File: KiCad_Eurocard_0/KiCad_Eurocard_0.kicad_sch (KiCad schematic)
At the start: 137 parts, among them IC1 ADF4351BCPZ, IC1 ADP3334ARZ, IC2 AD9959BCPZ, IC2 CY7C68013A-56LTX, J1 Conn_Coaxial, J2 Conn_Coaxial, J3 Conn_Coaxial, J4 Conn_Coaxial, J5 Conn_Coaxial, J6 Conn_Coaxial, J7 Conn_Coaxial, J8 Conn_Coaxial, J9 USB_B_Mini, SW1 SW_DIP_x01, SW2 SW_DIP_x01, U1 ADP150ACBZ-2.85R7, U2 ADP150ACBZ-2.85R7, U4 24LC64, Y1 ECS-240-12-20A-TR

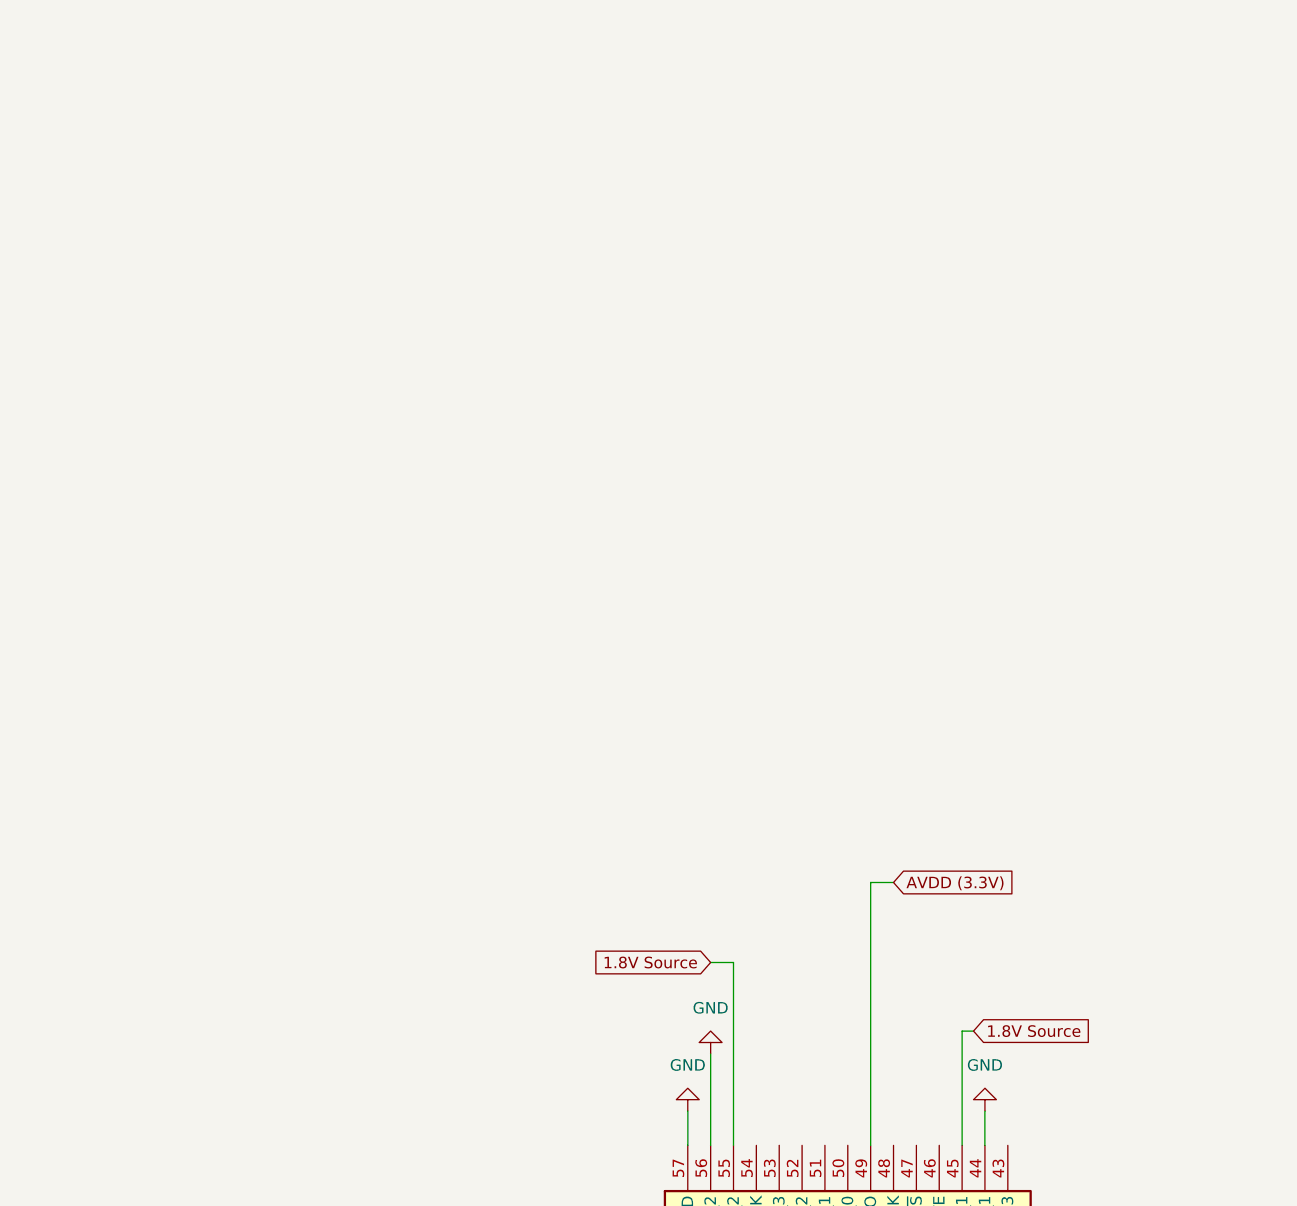
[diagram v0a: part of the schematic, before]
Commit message: Update KiCad_Eurocard_0.kicad_sch
test1000
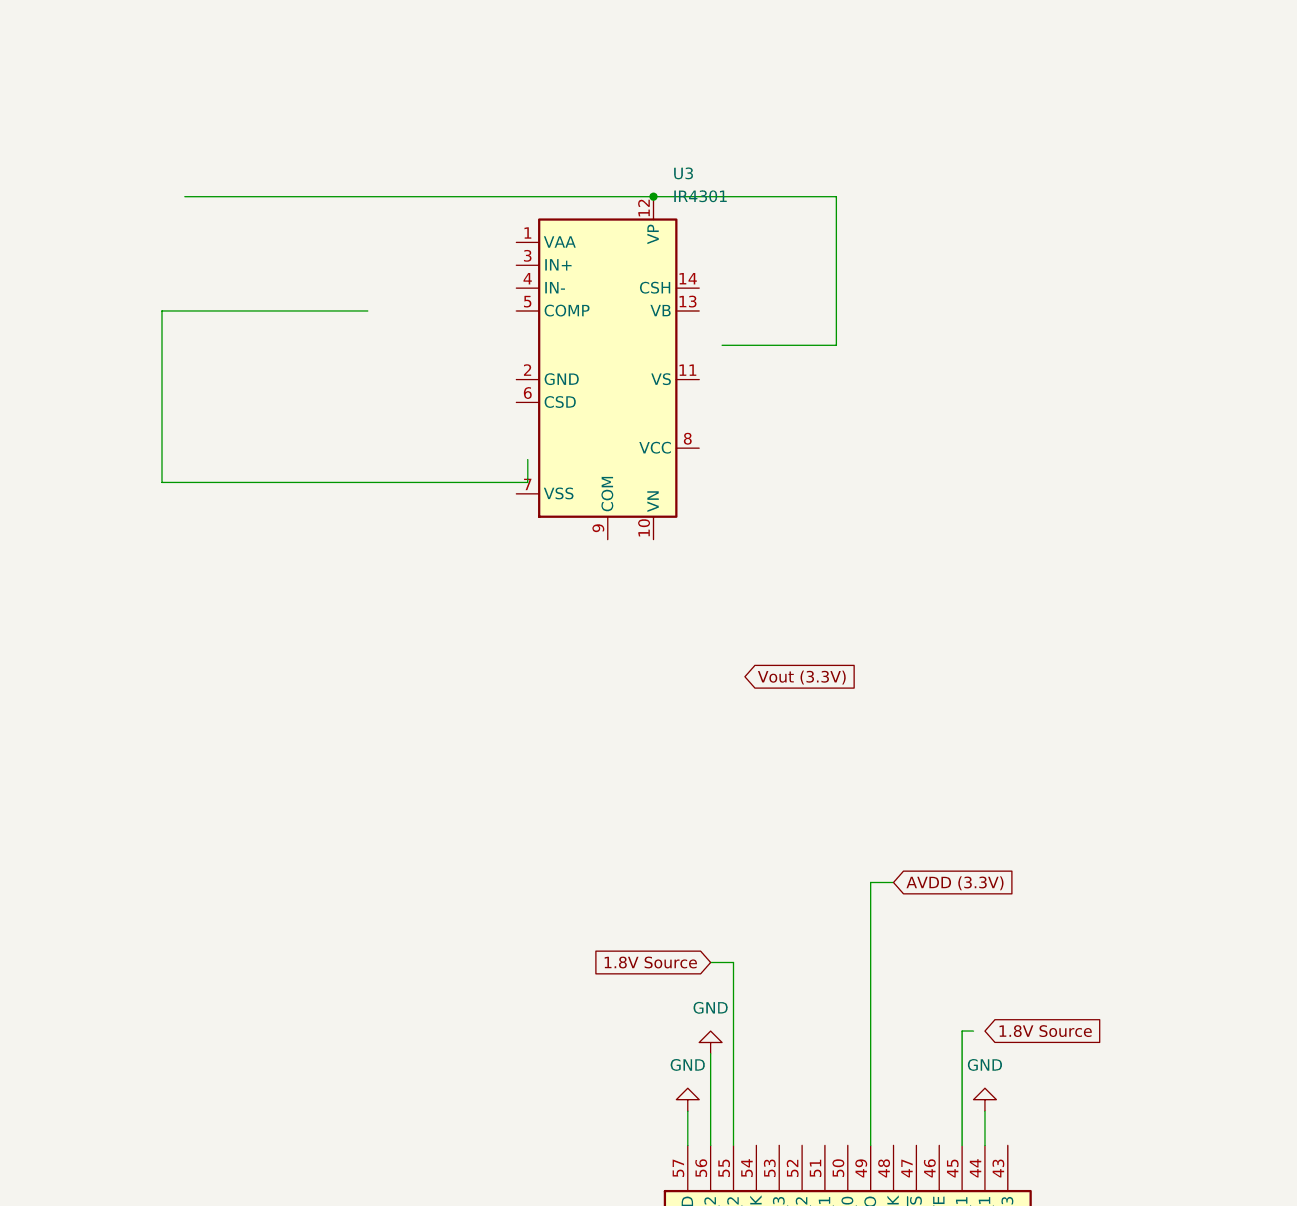
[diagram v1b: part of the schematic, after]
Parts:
- added U3: IR4301, Package_DFN_QFN:Infineon_PQFN-22-15-4EP_6x5mm_P0.65mm, symbol Amplifier_Audio:IR4301
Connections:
- net 1.8V Source: no longer IC2.45 (DVDD_1)
- new net: U3.15 (COM), U3.9 (COM)
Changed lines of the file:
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@@
 	)
 	(junction
+		(at 311.15 163.83)
+		(diameter 0)
+		(color 0 0 0 0)
+	)
+	(junction
 		(at 46.99 227.33)
 		(diameter 0)
@@
 	(wire
 		(pts
+			(xy 297.18 193.04) (xy 297.18 195.58)
+		)
+		(stroke
+			(width 0)
+			(type default)
+		)
+	)
+	(wire
+		(pts
 			(xy 306.07 367.03) (xy 306.07 368.3)
 		)
@@
 	(wire
 		(pts
+			(xy 279.4 176.53) (xy 256.54 176.53)
+		)
+		(stroke
+			(width 0)
+			(type default)
+		)
+	)
+	(wire
+		(pts
 			(xy 459.74 279.4) (xy 459.74 278.13)
 		)
@@
 	(wire
 		(pts
+			(xy 331.47 163.83) (xy 331.47 180.34)
+		)
+		(stroke
+			(width 0)
+			(type default)
+		)
+	)
+	(wire
+		(pts
 			(xy 115.57 107.95) (xy 128.27 107.95)
 		)
@@
 	(wire
 		(pts
+			(xy 256.54 176.53) (xy 256.54 195.58)
+		)
+		(stroke
+			(width 0)
+			(type default)
+		)
+	)
+	(wire
+		(pts
 			(xy 185.42 219.71) (xy 181.61 219.71)
 		)
@@
 	(wire
 		(pts
+			(xy 256.54 195.58) (xy 297.18 195.58)
+		)
+		(stroke
+			(width 0)
+			(type default)
+		)
+	)
+	(wire
+		(pts
 			(xy 85.09 227.33) (xy 85.09 234.95)
 		)
@@
 	(wire
 		(pts
+			(xy 311.15 163.83) (xy 331.47 163.83)
+		)
+		(stroke
+			(width 0)
+			(type default)
+		)
+	)
+	(wire
+		(pts
 			(xy 527.05 182.88) (xy 527.05 187.96)
 		)
@@
 	(wire
 		(pts
+			(xy 259.08 163.83) (xy 311.15 163.83)
+		)
+		(stroke
+			(width 0)
+			(type default)
+		)
+	)
+	(wire
+		(pts
 			(xy 485.14 22.86) (xy 499.11 22.86)
 		)
@@
 	(wire
 		(pts
+			(xy 318.77 180.34) (xy 331.47 180.34)
+		)
+		(stroke
+			(width 0)
+			(type default)
+		)
+	)
+	(wire
+		(pts
 			(xy 378.46 83.82) (xy 378.46 92.71)
 		)
@@
 		)
 	)
+	(global_label "Vout (3.3V)"
+		(shape input)
+		(at 321.31 217.17 0)
+		(fields_autoplaced yes)
+		(effects
+			(font
+				(size 1.27 1.27)
+			)
+			(justify left)
+		)
+		(property "Intersheetrefs" "${INTERSHEET_REFS}"
+			(at 335.1809 217.17 0)
+			(effects
+				(font
+					(size 1.27 1.27)
+				)
+				(justify left)
+				(hide yes)
+			)
+		)
+	)
 	(global_label "A2 OUT"
 		(shape input)
@@
 	(global_label "1.8V Source"
 		(shape input)
-		(at 346.71 256.54 0)
+		(at 347.98 256.54 0)
 		(fields_autoplaced yes)
 		(effects
@@
 		)
 		(property "Intersheetrefs" "${INTERSHEET_REFS}"
-			(at 361.2461 256.54 0)
+			(at 362.5161 256.54 0)
 			(effects
 				(font
@@
 		)
 		(instances
-			(project ""
+			(project "KiCad_Eurocard_0"
 				(path "/9cb3cf89-0e72-4eef-94e8-d924ebdf2eea"
 					(reference "IC1")
@@
 		)
 		(instances
-			(project ""
+			(project "KiCad_Eurocard_0"
 				(path "/9cb3cf89-0e72-4eef-94e8-d924ebdf2eea"
 					(reference "SW1")
@@
 		)
 		(instances
-			(project ""
+			(project "KiCad_Eurocard_0"
 				(path "/9cb3cf89-0e72-4eef-94e8-d924ebdf2eea"
 					(reference "#PWR06")
@@
 		)
 		(instances
-			(project ""
+			(project "KiCad_Eurocard_0"
 				(path "/9cb3cf89-0e72-4eef-94e8-d924ebdf2eea"
 					(reference "R39")
@@
 		)
 		(instances
-			(project ""
+			(project "KiCad_Eurocard_0"
 				(path "/9cb3cf89-0e72-4eef-94e8-d924ebdf2eea"
 					(reference "J9")
@@
 		)
 		(instances
-			(project ""
+			(project "KiCad_Eurocard_0"
 				(path "/9cb3cf89-0e72-4eef-94e8-d924ebdf2eea"
 					(reference "J1")
@@
 		)
 		(instances
-			(project ""
+			(project "KiCad_Eurocard_0"
 				(path "/9cb3cf89-0e72-4eef-94e8-d924ebdf2eea"
 					(reference "IC2")
@@
 		)
 		(instances
-			(project ""
+			(project "KiCad_Eurocard_0"
 				(path "/9cb3cf89-0e72-4eef-94e8-d924ebdf2eea"
 					(reference "#PWR035")
@@
 		)
 		(instances
-			(project ""
+			(project "KiCad_Eurocard_0"
 				(path "/9cb3cf89-0e72-4eef-94e8-d924ebdf2eea"
 					(reference "IC2")
@@
 		)
 		(instances
-			(project ""
+			(project "KiCad_Eurocard_0"
 				(path "/9cb3cf89-0e72-4eef-94e8-d924ebdf2eea"
 					(reference "D1")
@@
 		)
 		(instances
-			(project ""
+			(project "KiCad_Eurocard_0"
 				(path "/9cb3cf89-0e72-4eef-94e8-d924ebdf2eea"
 					(reference "Y1")
@@
 	)
 	(symbol
+		(lib_id "Amplifier_Audio:IR4301")
+		(at 306.07 184.15 0)
+		(unit 1)
+		(exclude_from_sim no)
+		(in_bom yes)
+		(on_board yes)
+		(dnp no)
+		(fields_autoplaced yes)
+		(property "Reference" "U3"
+			(at 313.2933 161.29 0)
+			(effects
+				(font
+					(size 1.27 1.27)
+				)
+				(justify left)
+			)
+		)
+		(property "Value" "IR4301"
+			(at 313.2933 163.83 0)
+			(effects
+				(font
+					(size 1.27 1.27)
+				)
+				(justify left)
+			)
+		)
+		(property "Footprint" "Package_DFN_QFN:Infineon_PQFN-22-15-4EP_6x5mm_P0.65mm"
+			(at 306.07 184.15 0)
+			(effects
+				(font
+					(size 1.27 1.27)
+					(italic yes)
+				)
+				(hide yes)
+			)
+		)
+		(property "Datasheet" "https://www.infineon.com/dgdl/ir4301.pdf?fileId=5546d462533600a4015355d5fc691819"
+			(at 306.07 184.15 0)
+			(effects
+				(font
+					(size 1.27 1.27)
+				)
+				(hide yes)
+			)
+		)
+		(property "Description" "PowIRaudio Integrated Analog Input Class D Audio Amplifier, 160W/4ohm, 80V, PQFN-22"
+			(at 306.07 184.15 0)
+			(effects
+				(font
+					(size 1.27 1.27)
+				)
+				(hide yes)
+			)
+		)
+		(pin "3"
+		)
+		(pin "1"
+		)
+		(pin "5"
+		)
+		(pin "6"
+		)
+		(pin "4"
+		)
+		(pin "2"
+		)
+		(pin "14"
+		)
+		(pin "8"
+		)
+		(pin "13"
+		)
+		(pin "11"
+		)
+		(pin "12"
+		)
+		(pin "7"
+		)
+		(pin "15"
+		)
+		(pin "9"
+		)
+		(pin "10"
+		)
+		(instances
+			(project "KiCad_Eurocard_0"
+				(path "/9cb3cf89-0e72-4eef-94e8-d924ebdf2eea"
+					(reference "U3")
+					(unit 1)
+				)
+			)
+		)
+	)
+	(symbol
 		(lib_id "power:GND")
 		(at 31.75 162.56 270)
@@
 		)
 		(instances
-			(project ""
+			(project "KiCad_Eurocard_0"
 				(path "/9cb3cf89-0e72-4eef-94e8-d924ebdf2eea"
 					(reference "S1")
@@
 		)
 		(instances
-			(project ""
+			(project "KiCad_Eurocard_0"
 				(path "/9cb3cf89-0e72-4eef-94e8-d924ebdf2eea"
 					(reference "R5")
@@
 		)
 		(instances
-			(project ""
+			(project "KiCad_Eurocard_0"
 				(path "/9cb3cf89-0e72-4eef-94e8-d924ebdf2eea"
 					(reference "C6")
@@
 		)
 		(instances
-			(project ""
+			(project "KiCad_Eurocard_0"
 				(path "/9cb3cf89-0e72-4eef-94e8-d924ebdf2eea"
 					(reference "U4")

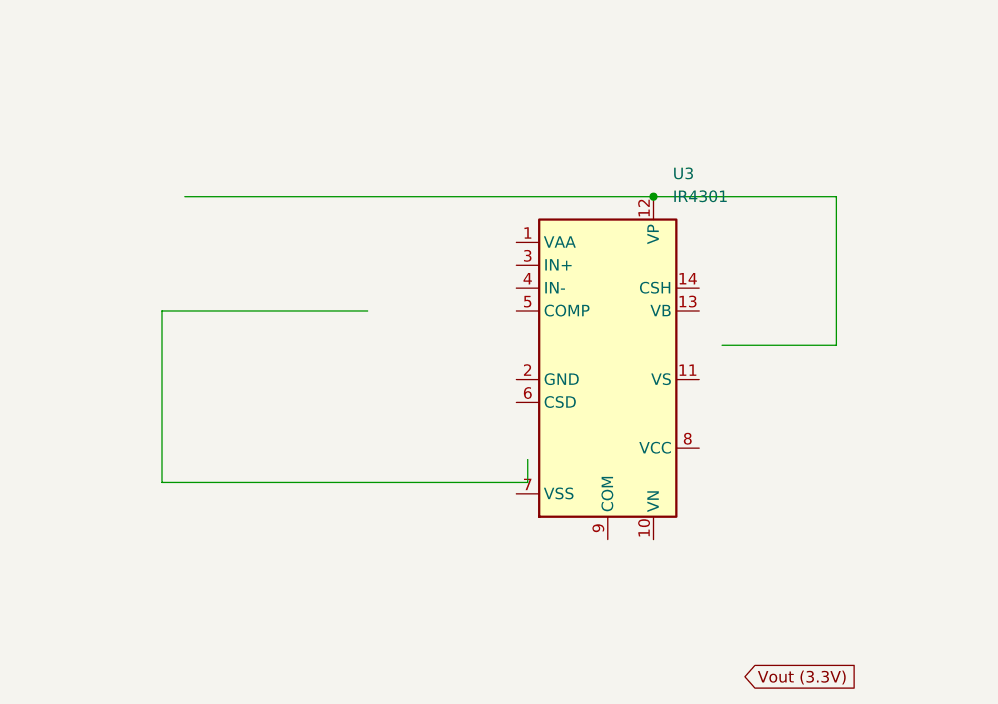
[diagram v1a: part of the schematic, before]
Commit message: Works now yay!
Works.
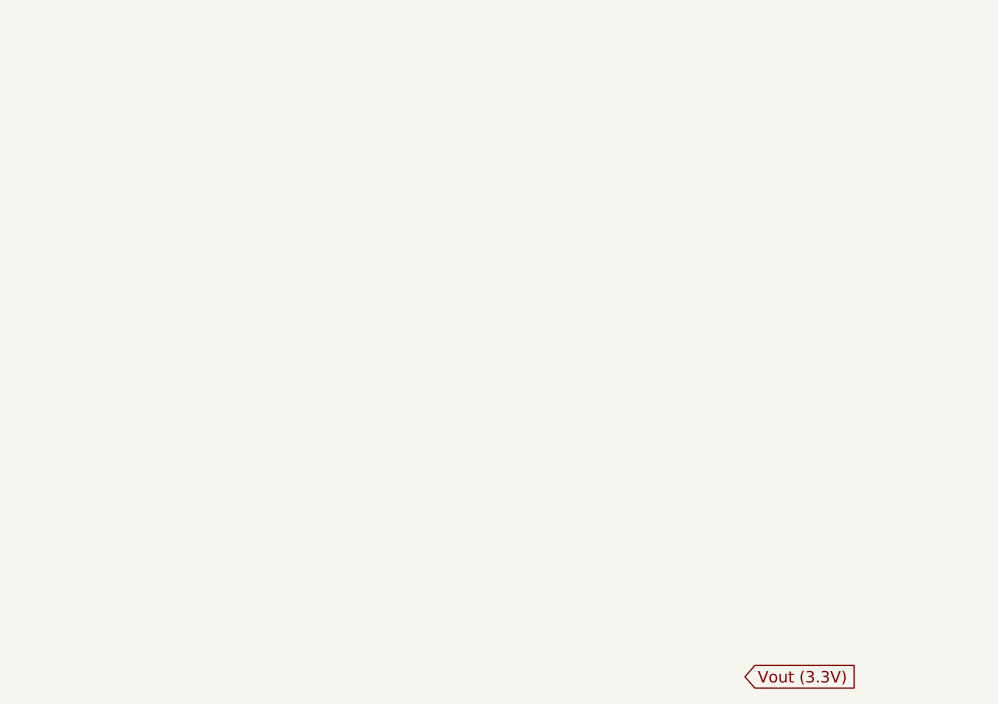
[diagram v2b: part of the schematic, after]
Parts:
- removed U3: IR4301, Package_DFN_QFN:Infineon_PQFN-22-15-4EP_6x5mm_P0.65mm, symbol Amplifier_Audio:IR4301
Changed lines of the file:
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@@
 	)
 	(junction
-		(at 311.15 163.83)
-		(diameter 0)
-		(color 0 0 0 0)
-	)
-	(junction
 		(at 46.99 227.33)
 		(diameter 0)
@@
 	(wire
 		(pts
-			(xy 297.18 193.04) (xy 297.18 195.58)
-		)
-		(stroke
-			(width 0)
-			(type default)
-		)
-	)
-	(wire
-		(pts
 			(xy 306.07 367.03) (xy 306.07 368.3)
 		)
@@
 	(wire
 		(pts
-			(xy 279.4 176.53) (xy 256.54 176.53)
-		)
-		(stroke
-			(width 0)
-			(type default)
-		)
-	)
-	(wire
-		(pts
 			(xy 459.74 279.4) (xy 459.74 278.13)
 		)
@@
 	(wire
 		(pts
-			(xy 331.47 163.83) (xy 331.47 180.34)
-		)
-		(stroke
-			(width 0)
-			(type default)
-		)
-	)
-	(wire
-		(pts
 			(xy 115.57 107.95) (xy 128.27 107.95)
 		)
@@
 	(wire
 		(pts
-			(xy 256.54 176.53) (xy 256.54 195.58)
-		)
-		(stroke
-			(width 0)
-			(type default)
-		)
-	)
-	(wire
-		(pts
 			(xy 185.42 219.71) (xy 181.61 219.71)
 		)
@@
 	(wire
 		(pts
-			(xy 256.54 195.58) (xy 297.18 195.58)
-		)
-		(stroke
-			(width 0)
-			(type default)
-		)
-	)
-	(wire
-		(pts
 			(xy 85.09 227.33) (xy 85.09 234.95)
 		)
@@
 	(wire
 		(pts
-			(xy 311.15 163.83) (xy 331.47 163.83)
-		)
-		(stroke
-			(width 0)
-			(type default)
-		)
-	)
-	(wire
-		(pts
 			(xy 527.05 182.88) (xy 527.05 187.96)
 		)
@@
 	(wire
 		(pts
-			(xy 259.08 163.83) (xy 311.15 163.83)
-		)
-		(stroke
-			(width 0)
-			(type default)
-		)
-	)
-	(wire
-		(pts
 			(xy 485.14 22.86) (xy 499.11 22.86)
 		)
@@
 	(wire
 		(pts
-			(xy 318.77 180.34) (xy 331.47 180.34)
-		)
-		(stroke
-			(width 0)
-			(type default)
-		)
-	)
-	(wire
-		(pts
 			(xy 378.46 83.82) (xy 378.46 92.71)
 		)
@@
 					(unit 1)
 				)
-			)
-		)
-	)
-	(symbol
-		(lib_id "Amplifier_Audio:IR4301")
-		(at 306.07 184.15 0)
-		(unit 1)
-		(exclude_from_sim no)
-		(in_bom yes)
-		(on_board yes)
-		(dnp no)
-		(fields_autoplaced yes)
-		(property "Reference" "U3"
-			(at 313.2933 161.29 0)
-			(effects
-				(font
-					(size 1.27 1.27)
-				)
-				(justify left)
-			)
-		)
-		(property "Value" "IR4301"
-			(at 313.2933 163.83 0)
-			(effects
-				(font
-					(size 1.27 1.27)
-				)
-				(justify left)
-			)
-		)
-		(property "Footprint" "Package_DFN_QFN:Infineon_PQFN-22-15-4EP_6x5mm_P0.65mm"
-			(at 306.07 184.15 0)
-			(effects
-				(font
-					(size 1.27 1.27)
-					(italic yes)
-				)
-				(hide yes)
-			)
-		)
-		(property "Datasheet" "https://www.infineon.com/dgdl/ir4301.pdf?fileId=5546d462533600a4015355d5fc691819"
-			(at 306.07 184.15 0)
-			(effects
-				(font
-					(size 1.27 1.27)
-				)
-				(hide yes)
-			)
-		)
-		(property "Description" "PowIRaudio Integrated Analog Input Class D Audio Amplifier, 160W/4ohm, 80V, PQFN-22"
-			(at 306.07 184.15 0)
-			(effects
-				(font
-					(size 1.27 1.27)
-				)
-				(hide yes)
-			)
-		)
-		(pin "3"
-		)
-		(pin "1"
-		)
-		(pin "5"
-		)
-		(pin "6"
-		)
-		(pin "4"
-		)
-		(pin "2"
-		)
-		(pin "14"
-		)
-		(pin "8"
-		)
-		(pin "13"
-		)
-		(pin "11"
-		)
-		(pin "12"
-		)
-		(pin "7"
-		)
-		(pin "15"
-		)
-		(pin "9"
-		)
-		(pin "10"
-		)
-		(instances
-			(project "KiCad_Eurocard_0"
-				(path "/9cb3cf89-0e72-4eef-94e8-d924ebdf2eea"
-					(reference "U3")
-					(unit 1)
-				)

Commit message: test
test again
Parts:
- C35: footprint (none) -> Capacitor_SMD:C_0201_0603Metric
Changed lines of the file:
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@@
 			)
 		)
-		(property "Footprint" ""
+		(property "Footprint" "Capacitor_SMD:C_0201_0603Metric"
 			(at 53.0352 372.11 0)
 			(effects
